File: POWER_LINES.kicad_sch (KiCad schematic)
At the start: 50 parts, among them J11 1717020, J12 1717020, J6 1730405, J8 1717020, J9 1717020, K3 G2R-1A-E DC5, K4 G2R-1A-E DC5, K5 G2R-1A-E DC5, K6 G2R-1A-E DC5, Q3 AO3400A, Q4 AO3400A

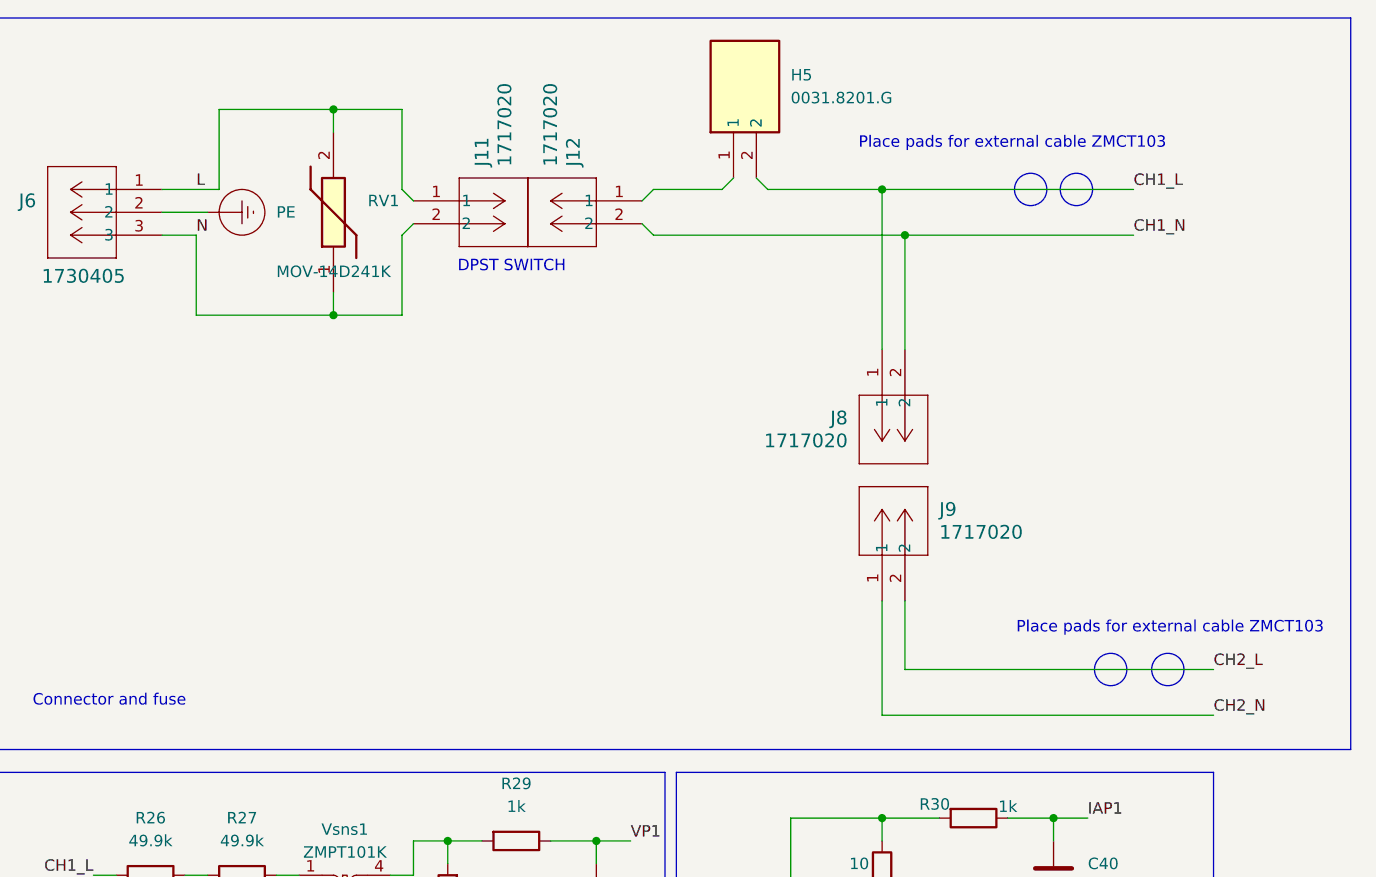
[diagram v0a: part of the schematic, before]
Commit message: MOV2
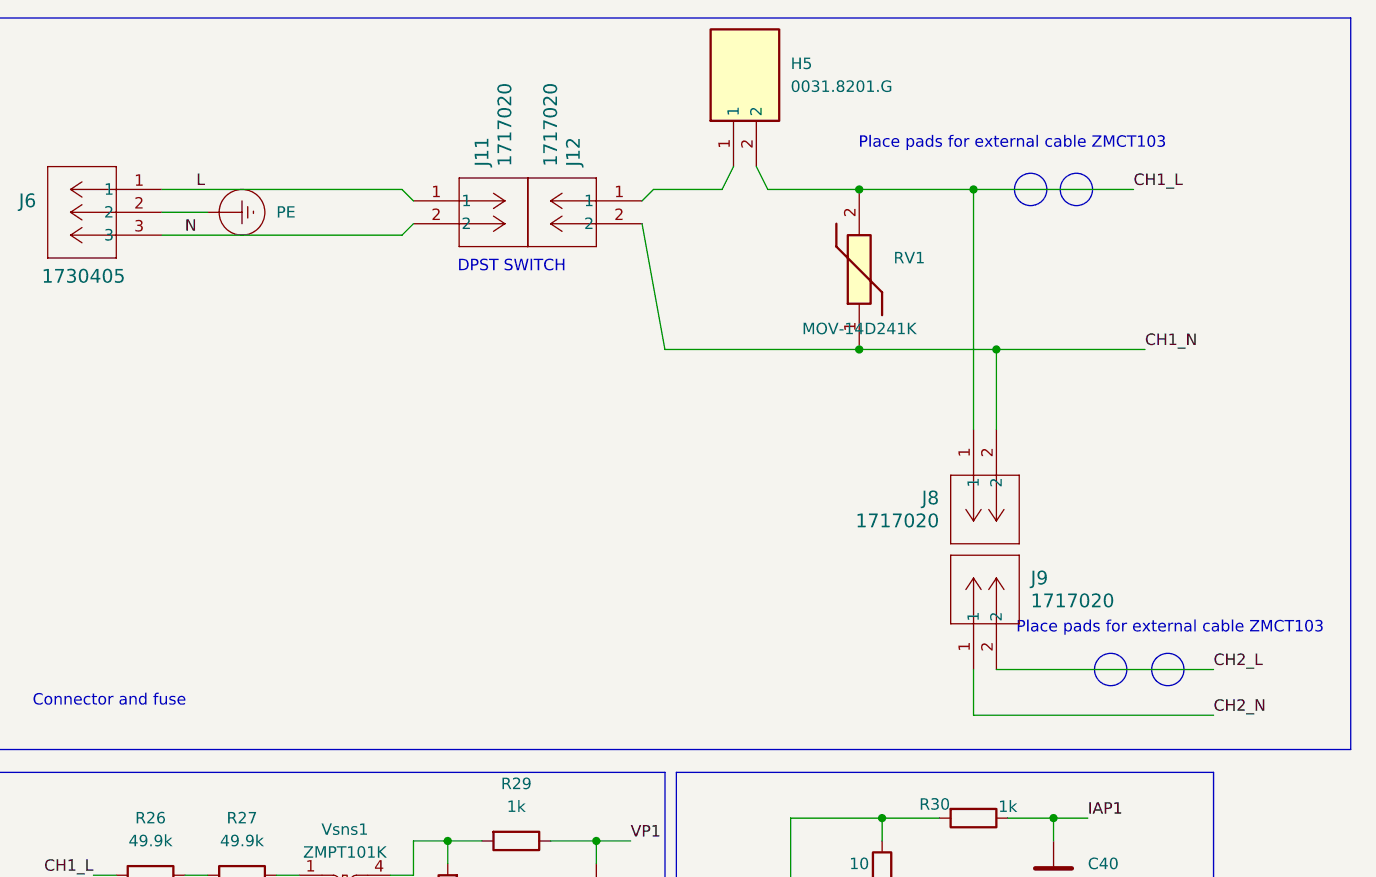
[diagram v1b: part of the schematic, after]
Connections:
- net CH1_L: now also RV1.2
- net CH1_N: now also RV1.1
- net L: no longer RV1.2
- net N: no longer RV1.1
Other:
- moved on the sheet: H5, J8, J9
